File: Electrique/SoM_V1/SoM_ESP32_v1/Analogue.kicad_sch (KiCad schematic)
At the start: 3 parts, among them U401 MCP4822, U402 MCP3202

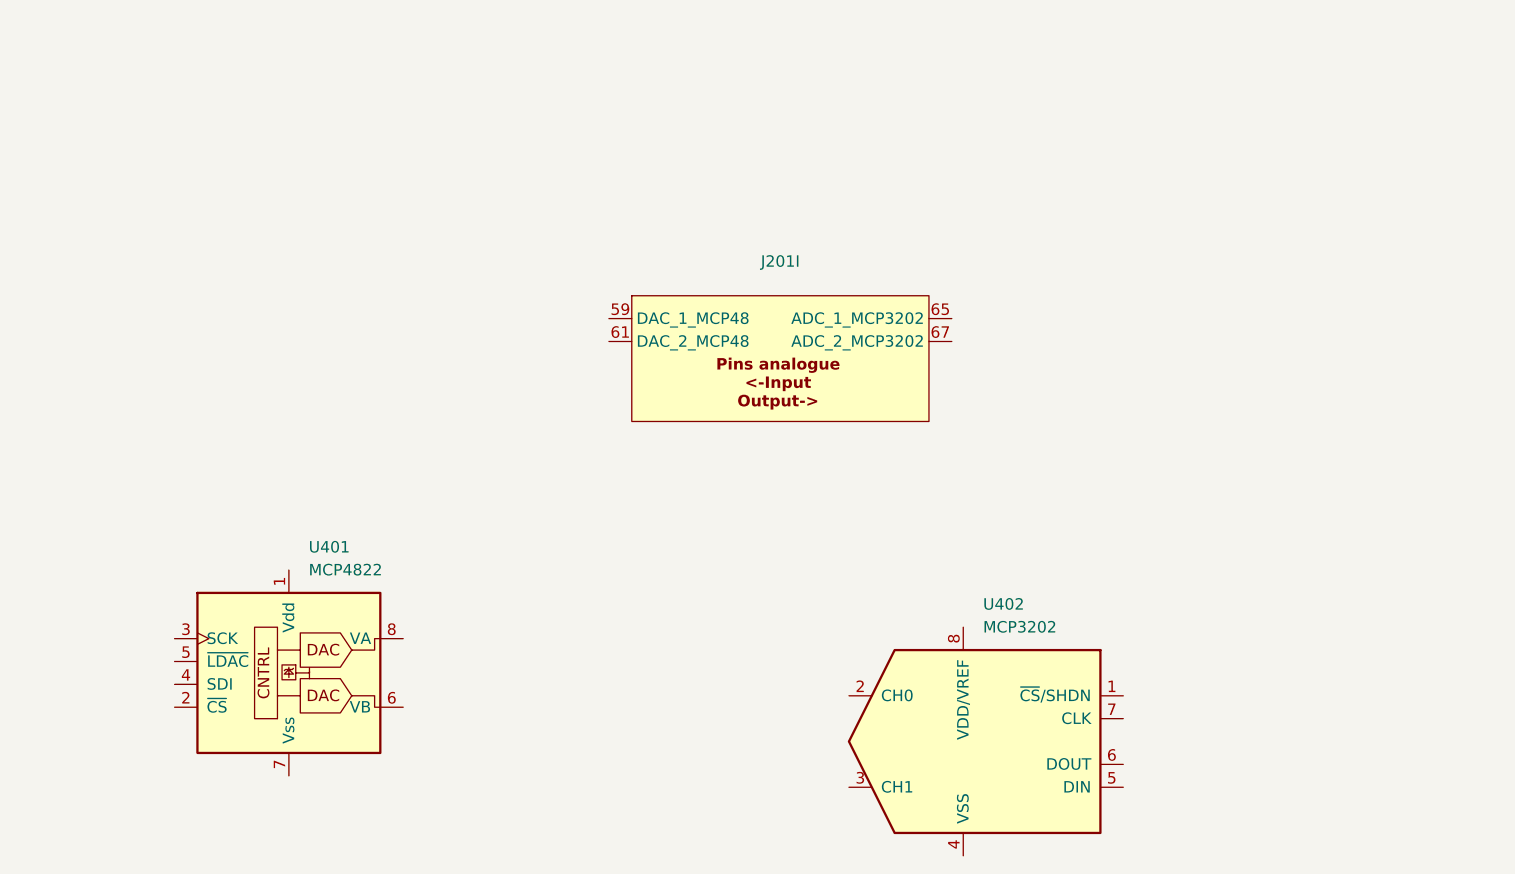
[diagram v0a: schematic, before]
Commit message: push pcb
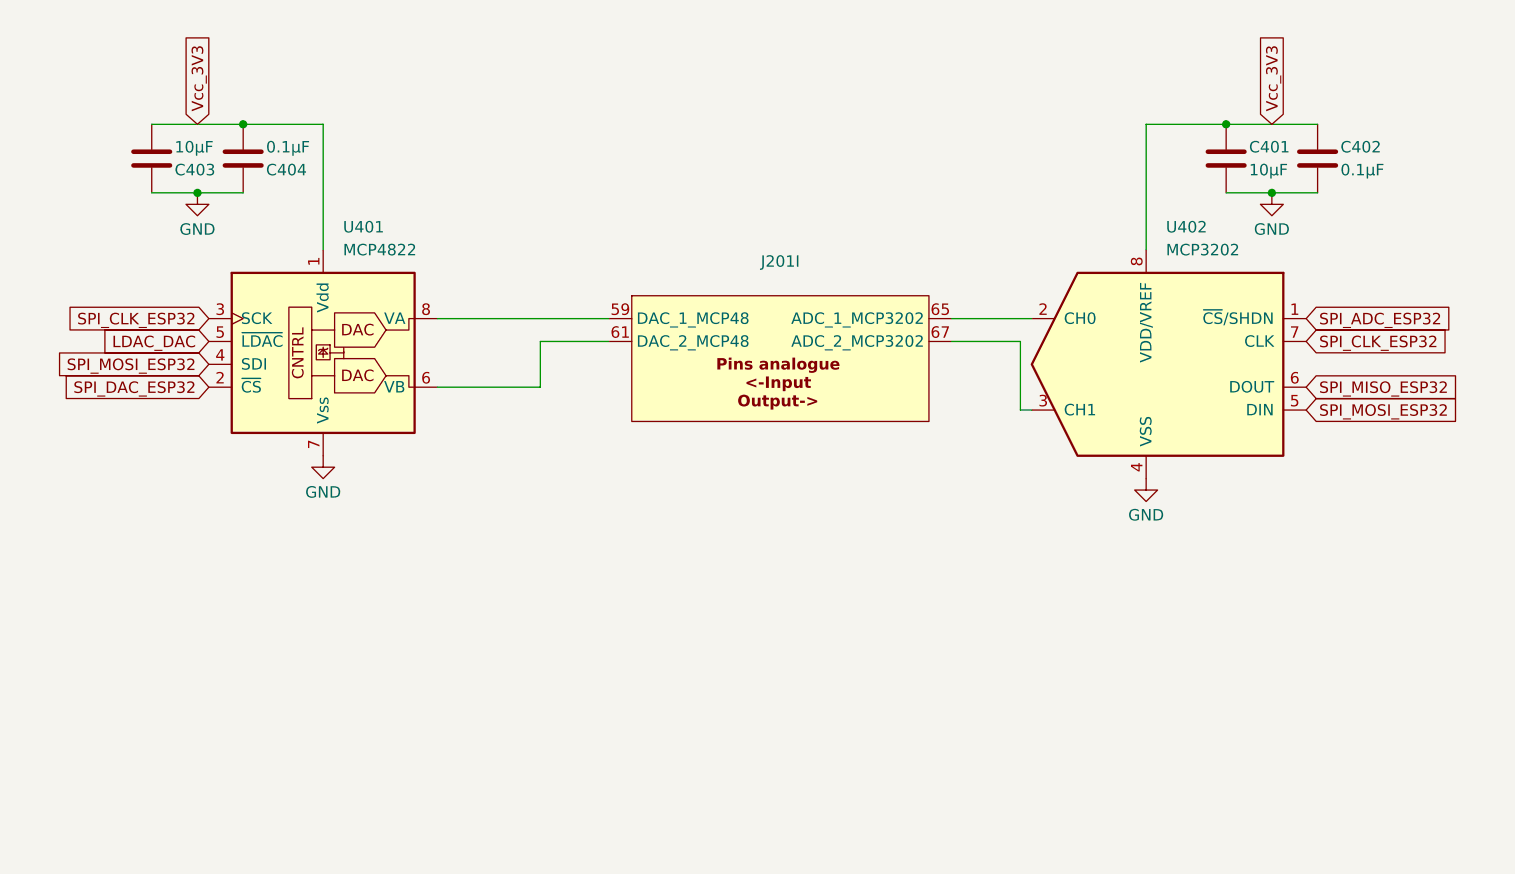
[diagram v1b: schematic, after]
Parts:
- added C401, C403: 10µF, Resistor_SMD:R_0805_2012Metric, symbol Device:C
- added C402, C404: 0.1µF, Resistor_SMD:R_0805_2012Metric, symbol Device:C
- U401, U402: footprint (none) -> Package_SO:SOIC-8_3.9x4.9mm_P1.27mm
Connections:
- net Vcc_3V3: now reaches U401.1 (Vdd)
- net Vcc_3V3: now also U402.8 (VDD/VREF), C401.1, C402.1, C403.2, C404.2
- net SPI_DAC_ESP32: now reaches U401.2 (~{CS})
- net SPI_CLK_ESP32: now reaches U401.3 (SCK)
- net SPI_CLK_ESP32: now also U402.7 (CLK)
- net SPI_MOSI_ESP32: now reaches U401.4 (SDI)
- net SPI_MOSI_ESP32: now also U402.5 (DIN)
- net LDAC_DAC: now reaches U401.5 (~{LDAC})
- net at U401.6 (VB): now also J201.61 (DAC_2_MCP48)
- net GND: now reaches U401.7 (Vss)
- net GND: now also U402.4 (VSS), C401.2, C402.2, C403.1, C404.1
- net at U401.8 (VA): now also J201.59 (DAC_1_MCP48)
- net at J201.65 (ADC_1_MCP3202): now also U402.2 (CH0)
- net at J201.67 (ADC_2_MCP3202): now also U402.3 (CH1)
- net SPI_ADC_ESP32: now reaches U402.1 (~{CS}/SHDN)
- net SPI_MISO_ESP32: now reaches U402.6 (DOUT)
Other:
- moved on the sheet: U401, U402
